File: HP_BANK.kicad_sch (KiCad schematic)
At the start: 2 parts, among them J6 DF40HC(3.0)-120DS, J7 DF40HC(3.0)-120DS

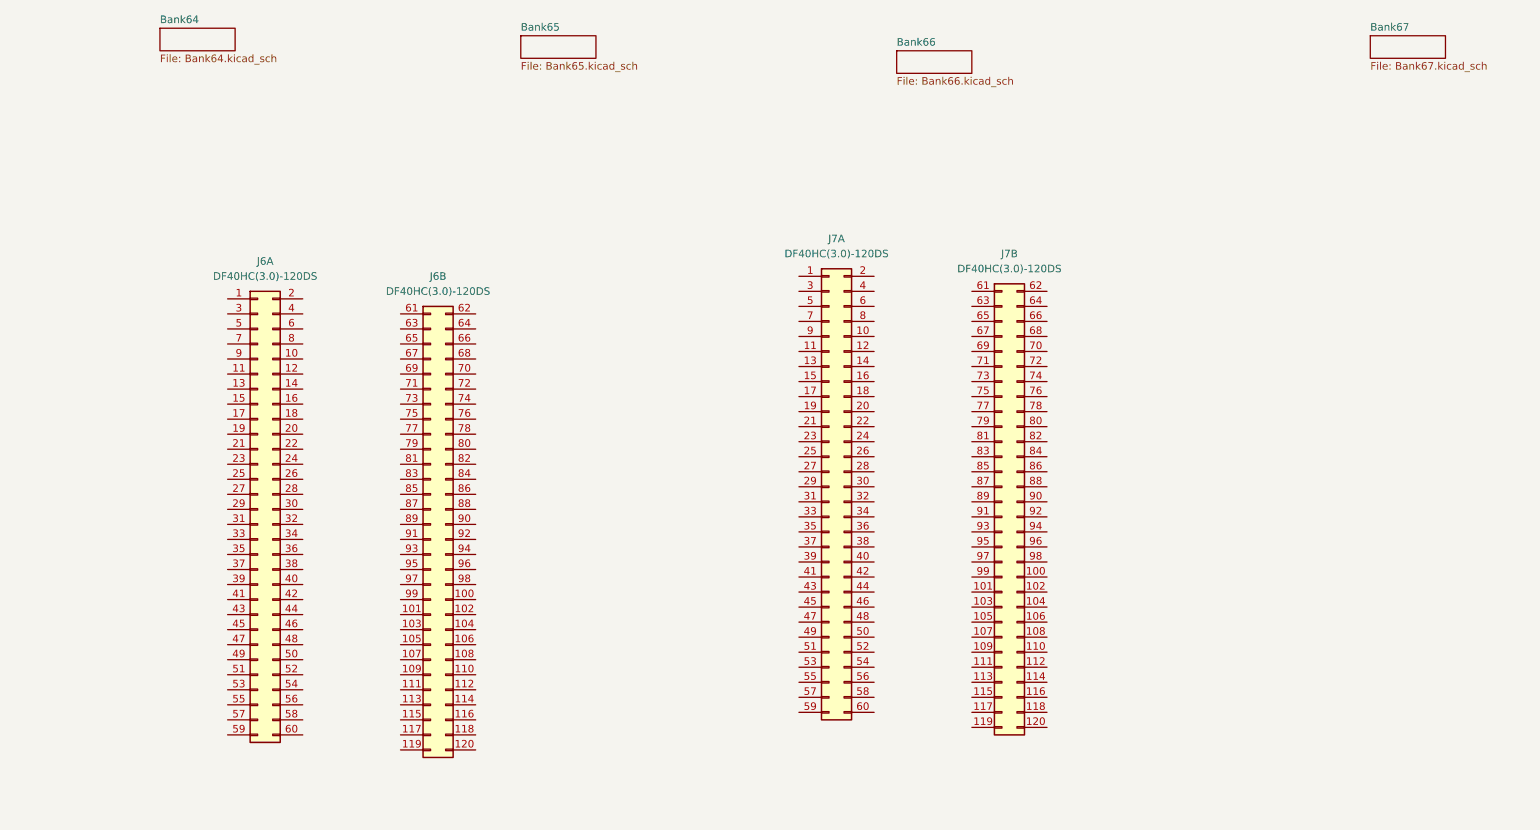
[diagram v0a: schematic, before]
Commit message: finishing schematic
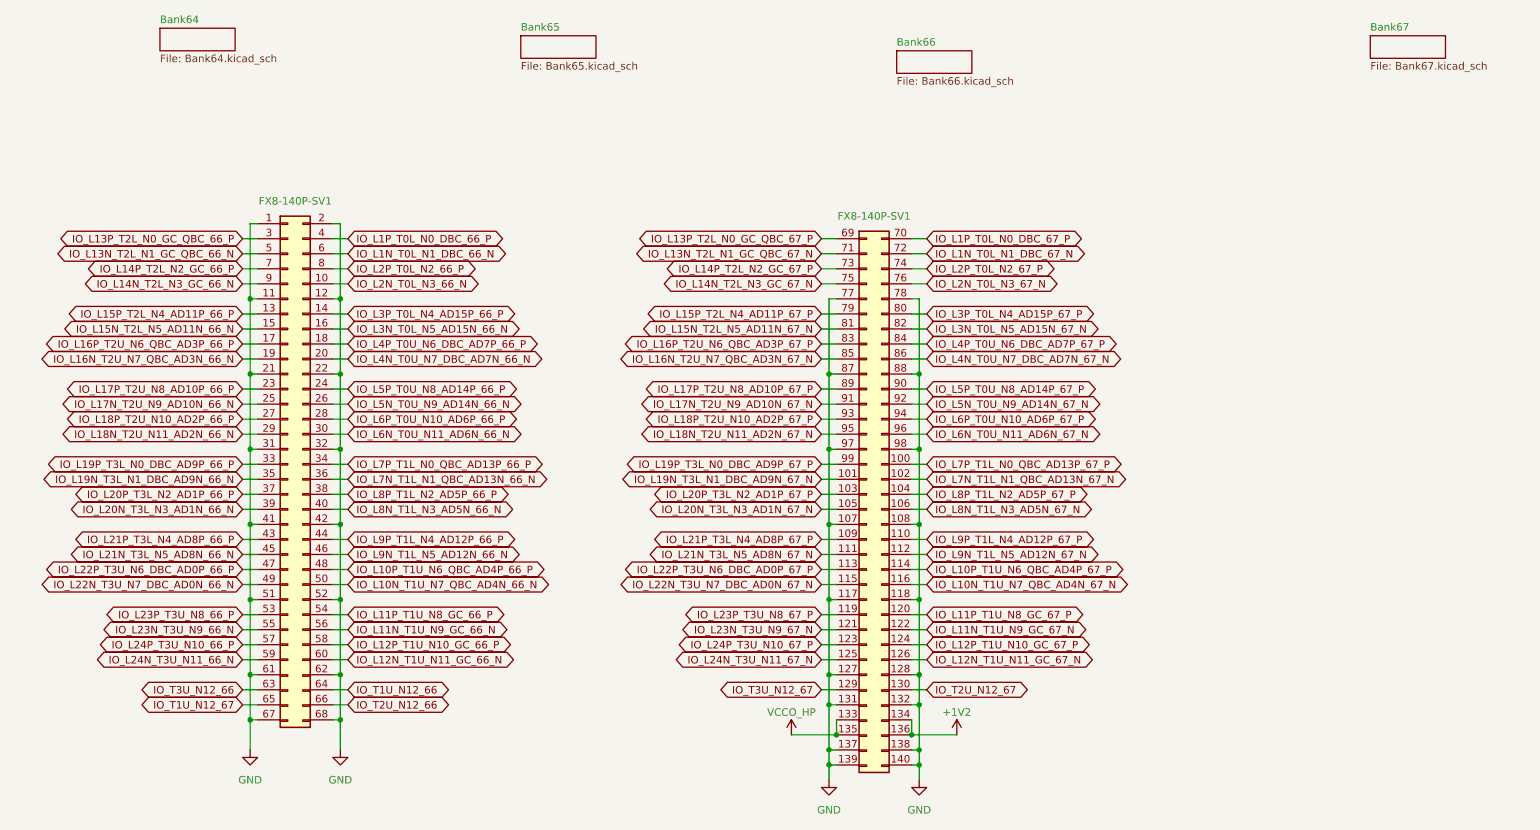
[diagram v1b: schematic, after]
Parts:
- removed J6, J7: DF40HC(3.0)-120DS, Connector_Hirose_DF40:Hirose_DF40C-120DS-0.4V_2x60_P0.4mm, symbol dfdtc_Connector:Conn_02x60_Odd_Even
- added J7: FX8-140P-SV1, Connector_Hirose_FX8:Hirose_FX8-140P-SV_2x70_P0.6mm, symbol dfdtc_Connector:Conn_02x70_Odd_Even
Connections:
- new net +1V2: J7.134, J7.136
- new net GND: J7.1 (Pin_1), J7.107 (Pin_107), J7.108 (Pin_108), J7.11 (Pin_11), J7.117 (Pin_117), J7.118 (Pin_118), J7.12 (Pin_12), J7.127, J7.128, J7.131, J7.132, J7.137, J7.138, J7.139, J7.140, J7.2 (Pin_2), J7.21 (Pin_21), J7.22 (Pin_22), J7.31 (Pin_31), J7.32 (Pin_32), J7.41 (Pin_41), J7.42 (Pin_42), J7.51 (Pin_51), J7.52 (Pin_52), J7.61 (Pin_61), J7.62 (Pin_62), J7.67 (Pin_67), J7.68 (Pin_68), J7.77 (Pin_77), J7.78 (Pin_78), J7.87 (Pin_87), J7.88 (Pin_88), J7.97 (Pin_97), J7.98 (Pin_98)
- new net IO_L10N_T1U_N7_QBC_AD4N_66_N: J7.50 (Pin_50)
- new net IO_L10N_T1U_N7_QBC_AD4N_67_N: J7.116 (Pin_116)
- new net IO_L10P_T1U_N6_QBC_AD4P_66_P: J7.48 (Pin_48)
- new net IO_L10P_T1U_N6_QBC_AD4P_67_P: J7.114 (Pin_114)
- new net IO_L11N_T1U_N9_GC_66_N: J7.56 (Pin_56)
- new net IO_L11N_T1U_N9_GC_67_N: J7.122
- new net IO_L11P_T1U_N8_GC_66_P: J7.54 (Pin_54)
- new net IO_L11P_T1U_N8_GC_67_P: J7.120 (Pin_120)
- new net IO_L12N_T1U_N11_GC_66_N: J7.60 (Pin_60)
- new net IO_L12N_T1U_N11_GC_67_N: J7.126
- new net IO_L12P_T1U_N10_GC_66_P: J7.58 (Pin_58)
- new net IO_L12P_T1U_N10_GC_67_P: J7.124
- new net IO_L13N_T2L_N1_GC_QBC_66_N: J7.5 (Pin_5)
- new net IO_L13N_T2L_N1_GC_QBC_67_N: J7.71 (Pin_71)
- new net IO_L13P_T2L_N0_GC_QBC_66_P: J7.3 (Pin_3)
- new net IO_L13P_T2L_N0_GC_QBC_67_P: J7.69 (Pin_69)
- new net IO_L14N_T2L_N3_GC_66_N: J7.9 (Pin_9)
- new net IO_L14N_T2L_N3_GC_67_N: J7.75 (Pin_75)
- new net IO_L14P_T2L_N2_GC_66_P: J7.7 (Pin_7)
- new net IO_L14P_T2L_N2_GC_67_P: J7.73 (Pin_73)
- new net IO_L15N_T2L_N5_AD11N_66_N: J7.15 (Pin_15)
- new net IO_L15N_T2L_N5_AD11N_67_N: J7.81 (Pin_81)
- new net IO_L15P_T2L_N4_AD11P_66_P: J7.13 (Pin_13)
- new net IO_L15P_T2L_N4_AD11P_67_P: J7.79 (Pin_79)
- new net IO_L16N_T2U_N7_QBC_AD3N_66_N: J7.19 (Pin_19)
- new net IO_L16N_T2U_N7_QBC_AD3N_67_N: J7.85 (Pin_85)
- new net IO_L16P_T2U_N6_QBC_AD3P_66_P: J7.17 (Pin_17)
- new net IO_L16P_T2U_N6_QBC_AD3P_67_P: J7.83 (Pin_83)
- new net IO_L17N_T2U_N9_AD10N_66_N: J7.25 (Pin_25)
- new net IO_L17N_T2U_N9_AD10N_67_N: J7.91 (Pin_91)
- new net IO_L17P_T2U_N8_AD10P_66_P: J7.23 (Pin_23)
- new net IO_L17P_T2U_N8_AD10P_67_P: J7.89 (Pin_89)
- new net IO_L18N_T2U_N11_AD2N_66_N: J7.29 (Pin_29)
- new net IO_L18N_T2U_N11_AD2N_67_N: J7.95 (Pin_95)
- new net IO_L18P_T2U_N10_AD2P_66_P: J7.27 (Pin_27)
- new net IO_L18P_T2U_N10_AD2P_67_P: J7.93 (Pin_93)
- new net IO_L19N_T3L_N1_DBC_AD9N_66_N: J7.35 (Pin_35)
- new net IO_L19N_T3L_N1_DBC_AD9N_67_N: J7.101 (Pin_101)
- new net IO_L19P_T3L_N0_DBC_AD9P_66_P: J7.33 (Pin_33)
- new net IO_L19P_T3L_N0_DBC_AD9P_67_P: J7.99 (Pin_99)
- new net IO_L1N_T0L_N1_DBC_66_N: J7.6 (Pin_6)
- new net IO_L1N_T0L_N1_DBC_67_N: J7.72 (Pin_72)
- new net IO_L1P_T0L_N0_DBC_66_P: J7.4 (Pin_4)
- new net IO_L1P_T0L_N0_DBC_67_P: J7.70 (Pin_70)
- new net IO_L20N_T3L_N3_AD1N_66_N: J7.39 (Pin_39)
- new net IO_L20N_T3L_N3_AD1N_67_N: J7.105 (Pin_105)
- new net IO_L20P_T3L_N2_AD1P_66_P: J7.37 (Pin_37)
- new net IO_L20P_T3L_N2_AD1P_67_P: J7.103 (Pin_103)
- new net IO_L21N_T3L_N5_AD8N_66_N: J7.45 (Pin_45)
- new net IO_L21N_T3L_N5_AD8N_67_N: J7.111 (Pin_111)
- new net IO_L21P_T3L_N4_AD8P_66_P: J7.43 (Pin_43)
- new net IO_L21P_T3L_N4_AD8P_67_P: J7.109 (Pin_109)
- new net IO_L22N_T3U_N7_DBC_AD0N_66_N: J7.49 (Pin_49)
- new net IO_L22N_T3U_N7_DBC_AD0N_67_N: J7.115 (Pin_115)
- new net IO_L22P_T3U_N6_DBC_AD0P_66_P: J7.47 (Pin_47)
- new net IO_L22P_T3U_N6_DBC_AD0P_67_P: J7.113 (Pin_113)
- new net IO_L23N_T3U_N9_66_N: J7.55 (Pin_55)
- new net IO_L23N_T3U_N9_67_N: J7.121
- new net IO_L23P_T3U_N8_66_P: J7.53 (Pin_53)
- new net IO_L23P_T3U_N8_67_P: J7.119 (Pin_119)
- new net IO_L24N_T3U_N11_66_N: J7.59 (Pin_59)
- new net IO_L24N_T3U_N11_67_N: J7.125
- new net IO_L24P_T3U_N10_66_P: J7.57 (Pin_57)
- new net IO_L24P_T3U_N10_67_P: J7.123
- new net IO_L2N_T0L_N3_66_N: J7.10 (Pin_10)
- new net IO_L2N_T0L_N3_67_N: J7.76 (Pin_76)
- new net IO_L2P_T0L_N2_66_P: J7.8 (Pin_8)
- new net IO_L2P_T0L_N2_67_P: J7.74 (Pin_74)
- new net IO_L3N_T0L_N5_AD15N_66_N: J7.16 (Pin_16)
- new net IO_L3N_T0L_N5_AD15N_67_N: J7.82 (Pin_82)
- new net IO_L3P_T0L_N4_AD15P_66_P: J7.14 (Pin_14)
- new net IO_L3P_T0L_N4_AD15P_67_P: J7.80 (Pin_80)
- new net IO_L4N_T0U_N7_DBC_AD7N_66_N: J7.20 (Pin_20)
- new net IO_L4N_T0U_N7_DBC_AD7N_67_N: J7.86 (Pin_86)
- new net IO_L4P_T0U_N6_DBC_AD7P_66_P: J7.18 (Pin_18)
- new net IO_L4P_T0U_N6_DBC_AD7P_67_P: J7.84 (Pin_84)
- new net IO_L5N_T0U_N9_AD14N_66_N: J7.26 (Pin_26)
- new net IO_L5N_T0U_N9_AD14N_67_N: J7.92 (Pin_92)
- new net IO_L5P_T0U_N8_AD14P_66_P: J7.24 (Pin_24)
- new net IO_L5P_T0U_N8_AD14P_67_P: J7.90 (Pin_90)
- new net IO_L6N_T0U_N11_AD6N_66_N: J7.30 (Pin_30)
- new net IO_L6N_T0U_N11_AD6N_67_N: J7.96 (Pin_96)
- new net IO_L6P_T0U_N10_AD6P_66_P: J7.28 (Pin_28)
- new net IO_L6P_T0U_N10_AD6P_67_P: J7.94 (Pin_94)
- new net IO_L7N_T1L_N1_QBC_AD13N_66_N: J7.36 (Pin_36)
- new net IO_L7N_T1L_N1_QBC_AD13N_67_N: J7.102 (Pin_102)
- new net IO_L7P_T1L_N0_QBC_AD13P_66_P: J7.34 (Pin_34)
- new net IO_L7P_T1L_N0_QBC_AD13P_67_P: J7.100 (Pin_100)
- new net IO_L8N_T1L_N3_AD5N_66_N: J7.40 (Pin_40)
- new net IO_L8N_T1L_N3_AD5N_67_N: J7.106 (Pin_106)
- new net IO_L8P_T1L_N2_AD5P_66_P: J7.38 (Pin_38)
- new net IO_L8P_T1L_N2_AD5P_67_P: J7.104 (Pin_104)
- new net IO_L9N_T1L_N5_AD12N_66_N: J7.46 (Pin_46)
- new net IO_L9N_T1L_N5_AD12N_67_N: J7.112 (Pin_112)
- new net IO_L9P_T1L_N4_AD12P_66_P: J7.44 (Pin_44)
- new net IO_L9P_T1L_N4_AD12P_67_P: J7.110 (Pin_110)
- new net IO_T1U_N12_66: J7.64 (Pin_64)
- new net IO_T1U_N12_67: J7.65 (Pin_65)
- new net IO_T2U_N12_66: J7.66 (Pin_66)
- new net IO_T2U_N12_67: J7.130
- new net IO_T3U_N12_66: J7.63 (Pin_63)
- new net IO_T3U_N12_67: J7.129
- new net VCCO_HP: J7.133, J7.135
